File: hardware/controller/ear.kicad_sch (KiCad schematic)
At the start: 25 parts, among them U6 EMS4000RSW, U7 baochip1x, Y2 48 MHz

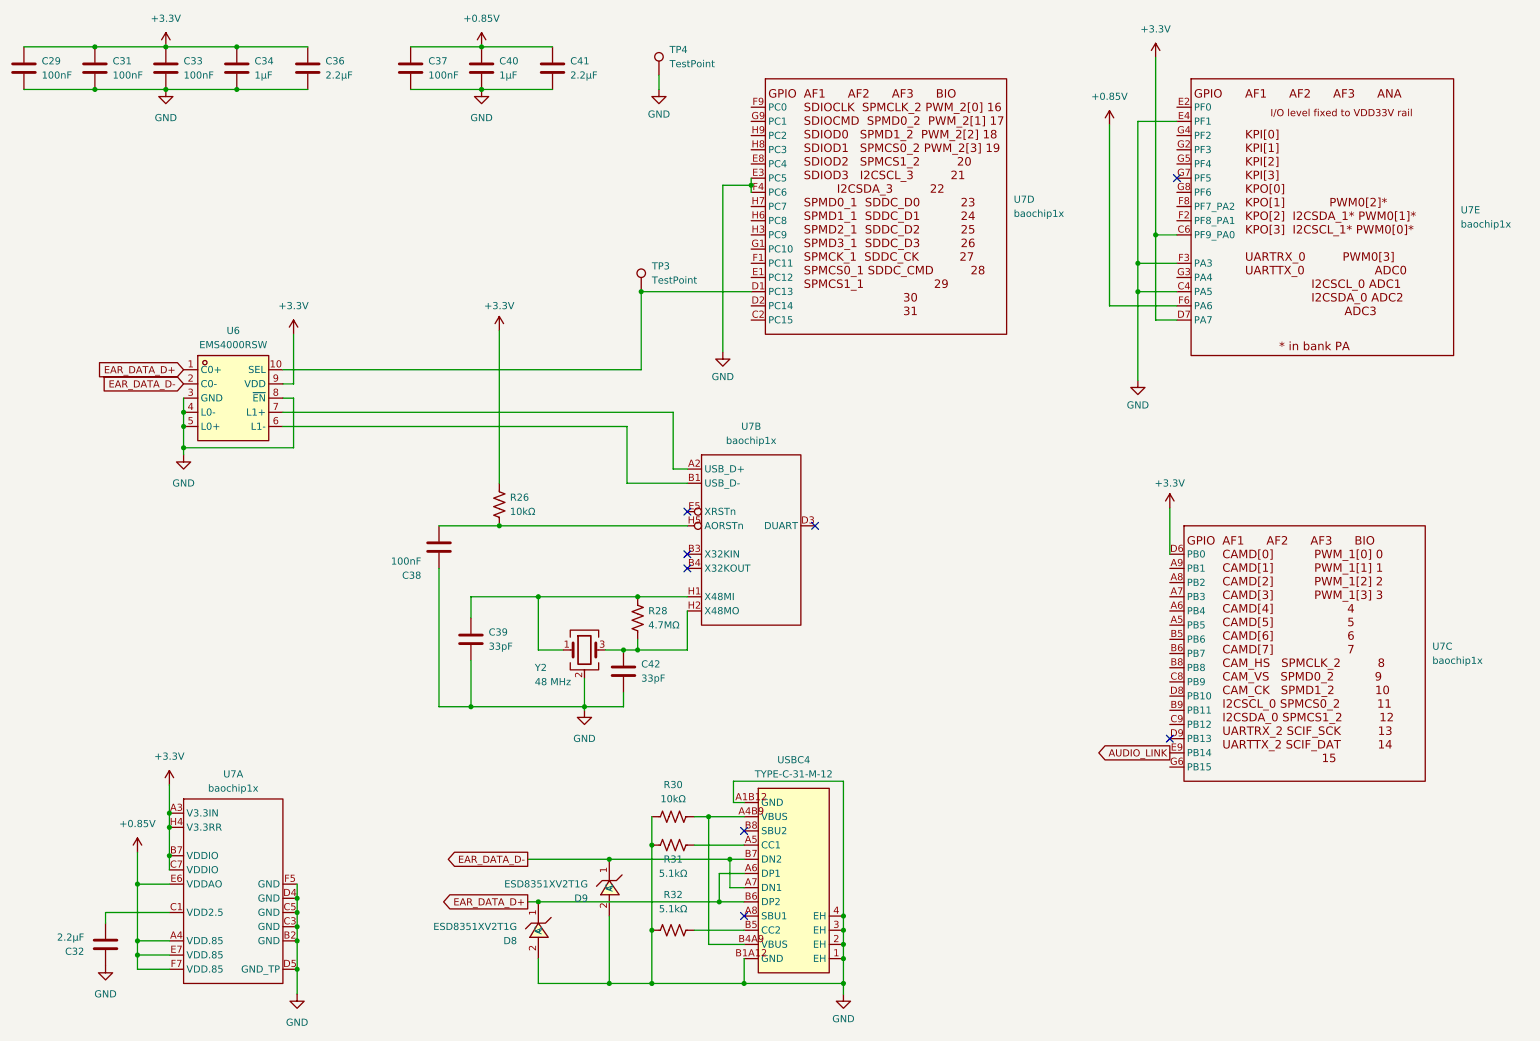
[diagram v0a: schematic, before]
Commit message: first round of schematic v3 done
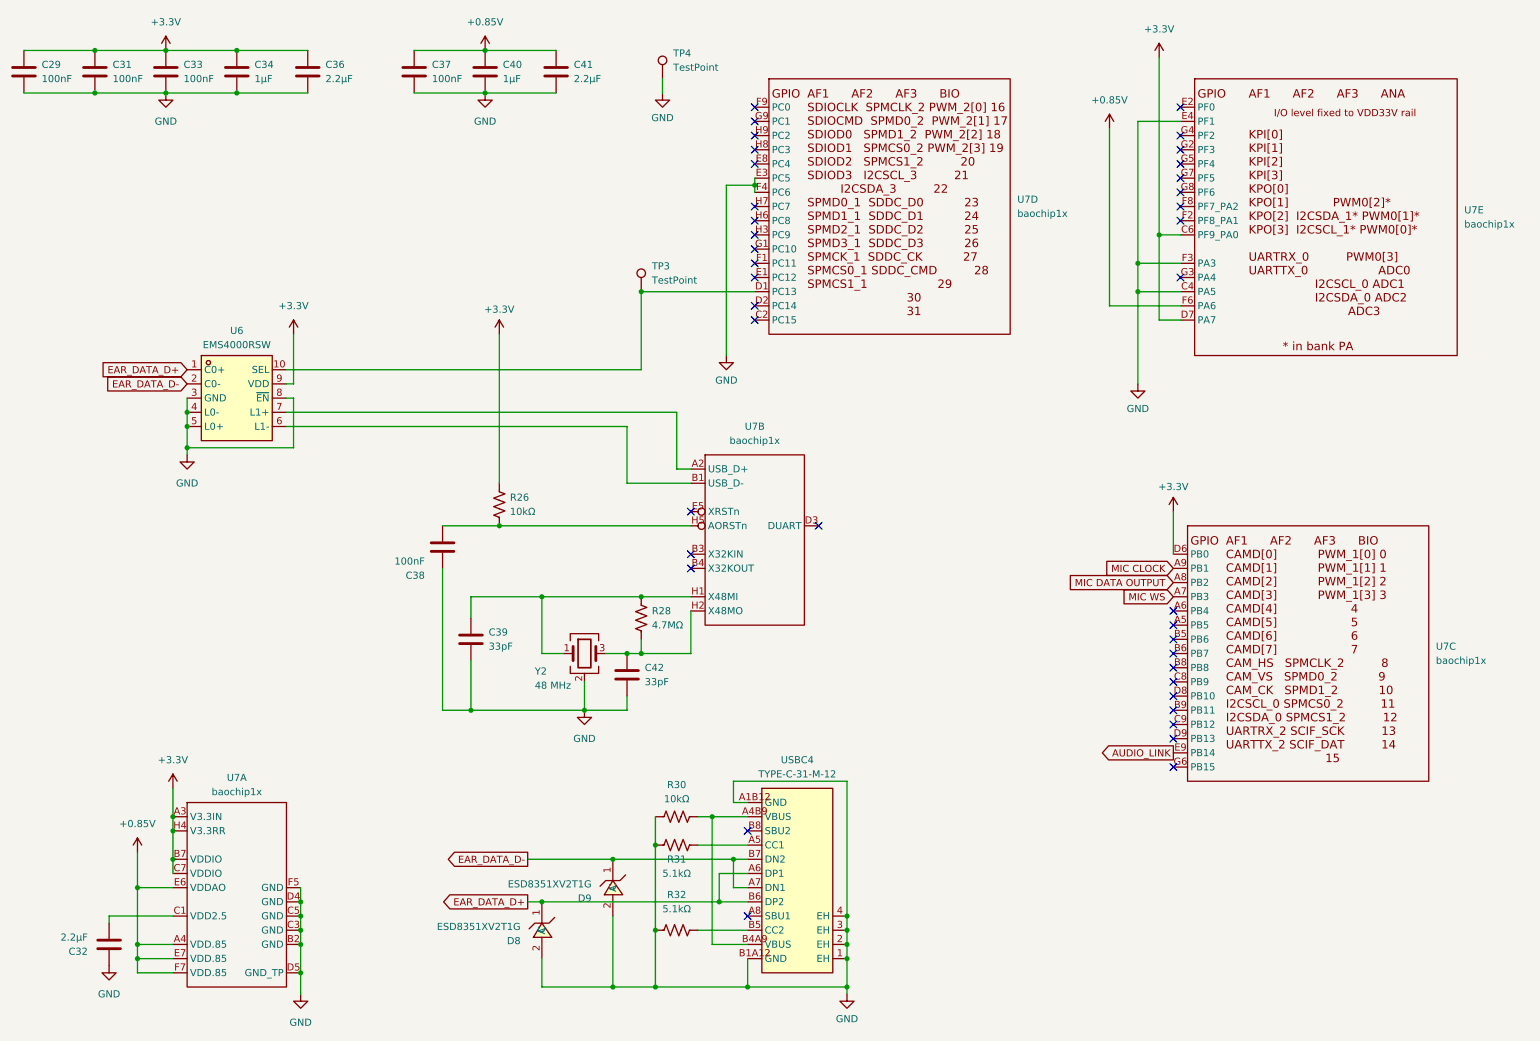
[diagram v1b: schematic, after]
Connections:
- net MIC WS: now reaches U7.A7 (PB3)
- net MIC DATA OUTPUT: now reaches U7.A8 (PB2)
- net MIC CLOCK: now reaches U7.A9 (PB1)
- no-connect marks 8 -> 39
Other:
- moved on the sheet: C29, C31, C32, C33, C34, C36, C37, C38, C40, C41, C42, D8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
